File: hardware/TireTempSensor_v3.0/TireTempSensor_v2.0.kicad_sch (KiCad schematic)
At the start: 36 parts, among them J2 CAN_01x04, J3 FTSH-107-01-L-D-K, SW1 RESET, SW2 3 pos dip switch, U1 STM32G0C1KCTxN, Y1 16MGHz

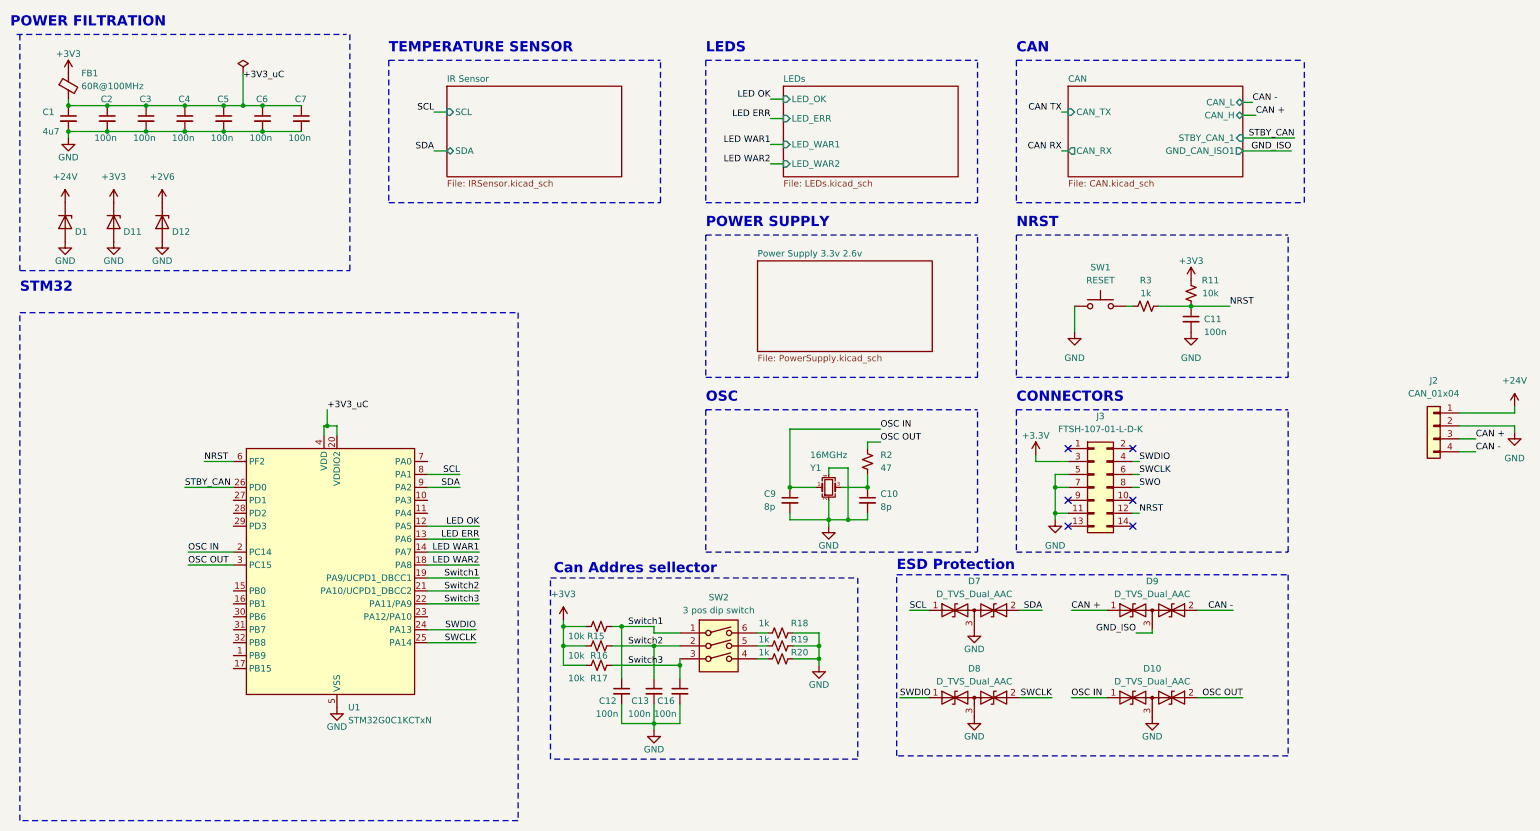
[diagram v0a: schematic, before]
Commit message: Poprawki, kontynuacja layoutu
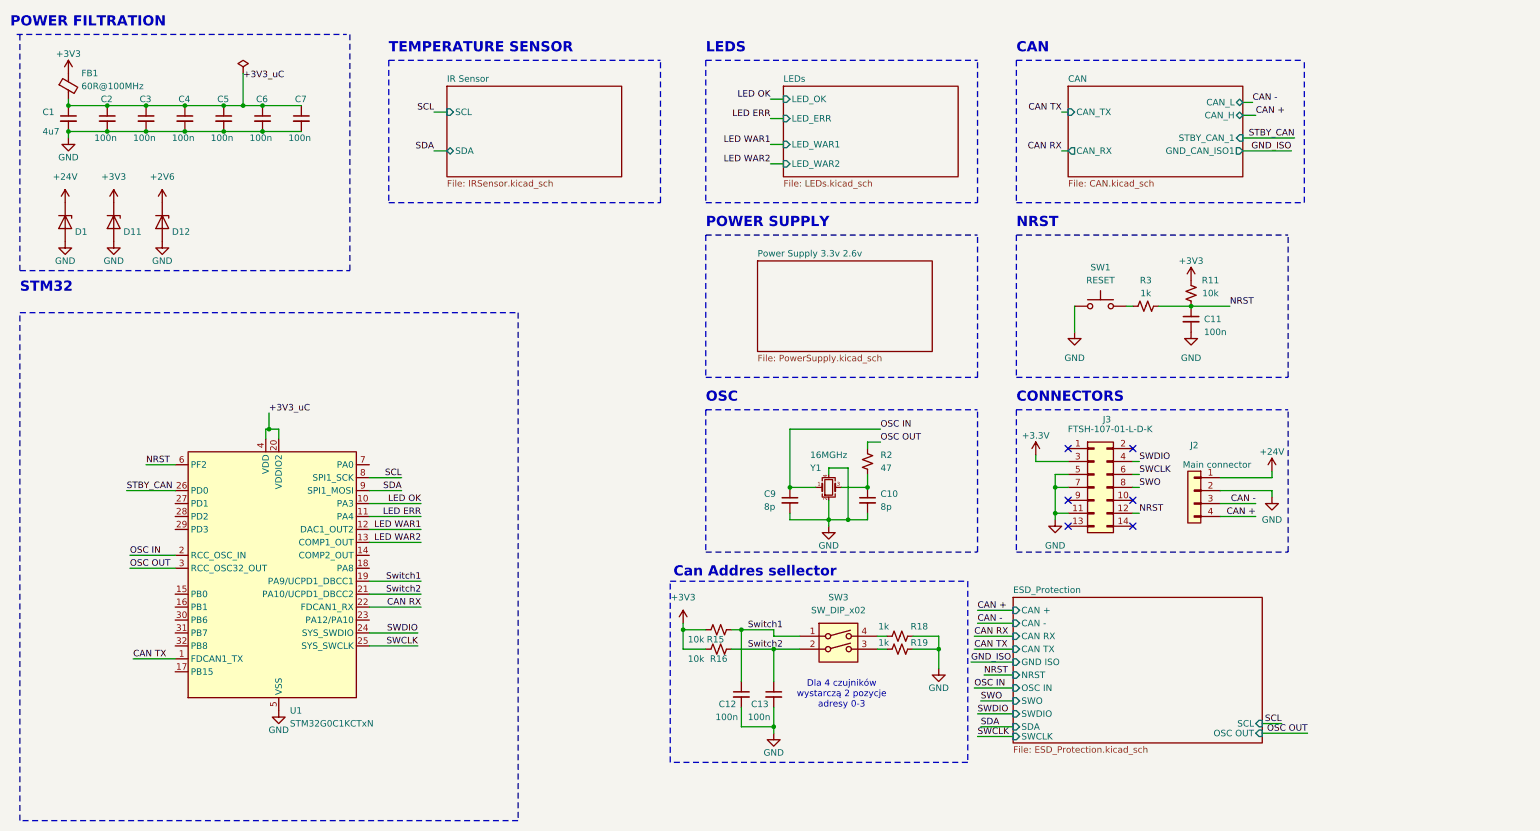
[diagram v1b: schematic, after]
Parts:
- removed C16: 100n, Capacitor_SMD:C_0603_1608Metric, symbol Device:C_Small
- removed D10, D7, D8, D9: D_TVS_Dual_AAC, Package_TO_SOT_SMD:SOT-23_Handsoldering, symbol Device:D_TVS_Dual_AAC
- removed R17: 10k, Resistor_SMD:R_0603_1608Metric, symbol Device:R_Small_US
- removed R20: 1k, Resistor_SMD:R_0603_1608Metric, symbol Device:R_Small_US
- removed SW2: 3 pos dip switch, footprint:DS04254103BKSMT, symbol Switch:SW_DIP_x03
- added SW3: SW_DIP_x02, footprint:2192LPST, symbol Switch:SW_DIP_x02
- J2: value CAN_01x04 -> Main connector; footprint Connector_Wire:SolderWire-0.1sqmm_1x04_P3.6mm_D0.4mm_OD1mm_Relief -> footprint:M80-51004YY
- J3: footprint Samacsys:FTSH-107-XX-YYY-D-K -> footprint:FTSH-107-XX-YYY-DV-K
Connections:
- net Switch3 is gone; now on net CAN RX: U1.22 (PA11/PA9)
- net CAN +: now also J2.4 (Pin_4); no longer J2.3 (Pin_3)
- net CAN -: now also J2.3 (Pin_3); no longer J2.4 (Pin_4)
- net CAN TX: now also U1.1 (PB9)
- net LED ERR: now also U1.11 (PA4); no longer U1.13 (PA6)
- net LED OK: now also U1.10 (PA3); no longer U1.12 (PA5)
- net LED WAR1: now also U1.12 (PA5); no longer U1.14 (PA7)
- net LED WAR2: now also U1.13 (PA6); no longer U1.18 (PA8)
- net Switch1: now also SW3.1
- net Switch2: now also SW3.2
- net at R19.1: now also SW3.3
- net at R18.1: now also SW3.4
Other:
- added sheet ESD_Protection (ESD_Protection.kicad_sch)
- note added: "Dla 4 czujników wystarczą 2 pozycje adresy 0-3"
- note removed: "ESD Protection"
- moved on the sheet: C12, C13, J2, R15, R16, R18, R19, U1
